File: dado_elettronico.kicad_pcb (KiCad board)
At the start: 2 copper layers, 29.4 x 23 mm, 29 parts, among them Q1 2N2219, SW1 SW_DIP_x01, U1 NE555P, U2 4017

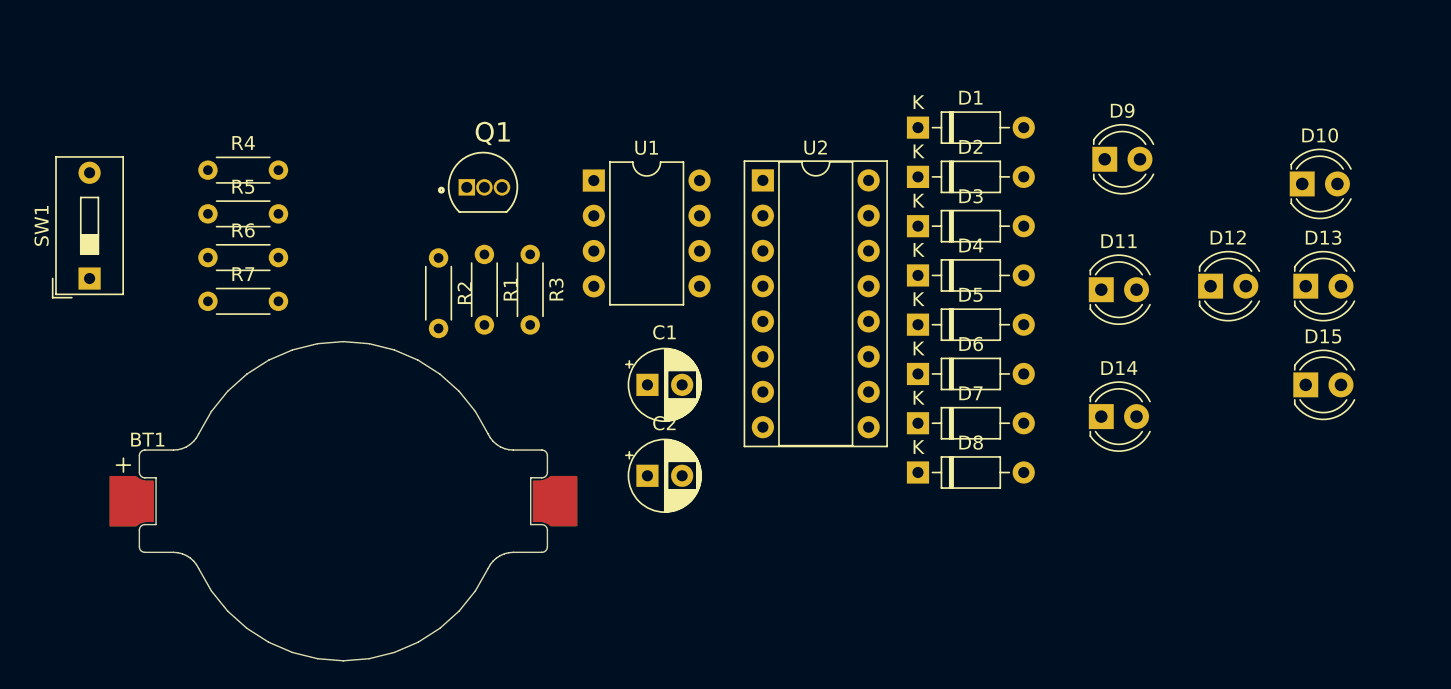
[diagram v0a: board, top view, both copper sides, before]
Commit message: sbroglio per test incisione
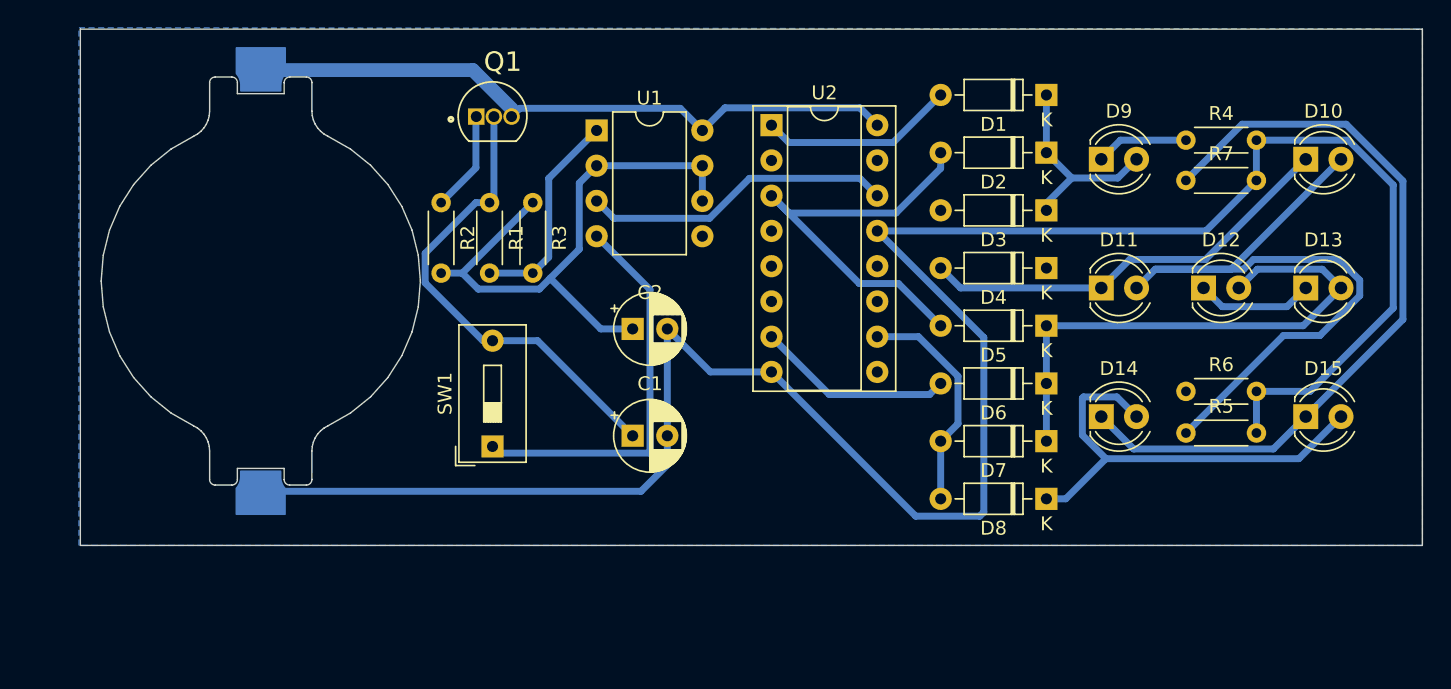
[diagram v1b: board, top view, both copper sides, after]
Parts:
- BT1: moved to B.Cu
- moved R5 72.2 mm to (149.9, 69.0)
- moved R6 71.1 mm to (149.9, 66.0)
- moved R7 71.0 mm to (149.9, 50.8)
- moved R4 70.5 mm to (149.9, 47.9)
- moved SW1 31.5 mm to (99.9, 70.0)
- moved BT1 16.9 mm to (83.2, 58.0), turned to -90 degrees
- moved C2 10.6 mm to (110.0, 61.5)
- moved D1 9.55 mm to (139.8, 44.6), turned to 180 degrees
- moved D8 9.45 mm to (139.8, 73.7), turned to 180 degrees
- moved D2 9.42 mm to (139.8, 48.8), turned to 180 degrees
- moved D7 9.34 mm to (139.8, 69.6), turned to 180 degrees
- moved D3 9.32 mm to (139.8, 53.0), turned to 180 degrees
- moved D6 9.28 mm to (139.8, 65.4), turned to 180 degrees
- moved D4 9.27 mm to (139.8, 57.1), turned to 180 degrees
- moved D5 9.25 mm to (139.8, 61.3), turned to 180 degrees
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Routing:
- net GND: track 0.00 -> 174.2 mm
- net Vcc: track 0.00 -> 76.7 mm
- net Net-(D14-K): track 0.00 -> 55.6 mm
- net Net-(D10-A): track 0.00 -> 51.9 mm
- net dis: track 0.00 -> 43.0 mm
- net Net-(D12-A): track 0.00 -> 39.2 mm
- net Net-(Q1-B): track 0.00 -> 34.1 mm
- net Net-(D14-A): track 0.00 -> 33.3 mm
- net Q0: track 0.00 -> 31.2 mm
- net Net-(D10-K): track 0.00 -> 30.7 mm
- net Net-(U1-Q): track 0.00 -> 22.4 mm
- net Q4: track 0.00 -> 16.4 mm
- net Net-(D1-K): track 0.00 -> 15.1 mm
- net Q3: track 0.00 -> 14.2 mm
- net Q5: track 0.00 -> 14.1 mm
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- added copper zone on B.Cu, net GND
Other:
- board size 29.4 x 23 mm -> 96.7 x 37.2 mm
